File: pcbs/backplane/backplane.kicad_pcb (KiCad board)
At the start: 2 copper layers, 80 x 50 mm, 39 parts, among them P1 USB_B, P2 CONN_01X10, P3 CONN_02X03, P4 CONN_02X03, P5 CONN_02X07, P6 CONN_02X07, P7 CONN_01X03, P8 CONN_01X03, Q1 MMBT3904, Q2 MMBT3904, U1 LM358, U2 TC1262-33VDB, U3 LM358, U4 CH340G, Y1 Crystal

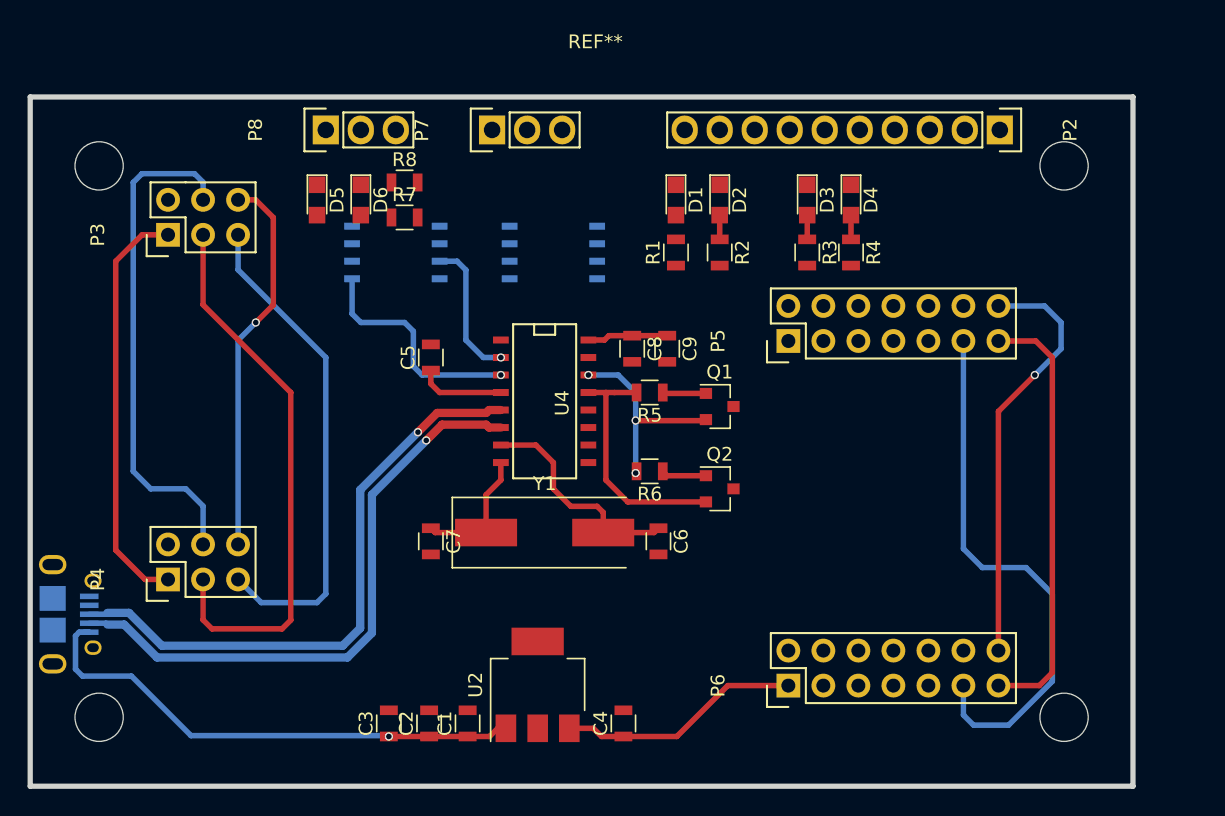
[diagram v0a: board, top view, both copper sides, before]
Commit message: Backplane version 1 ready.
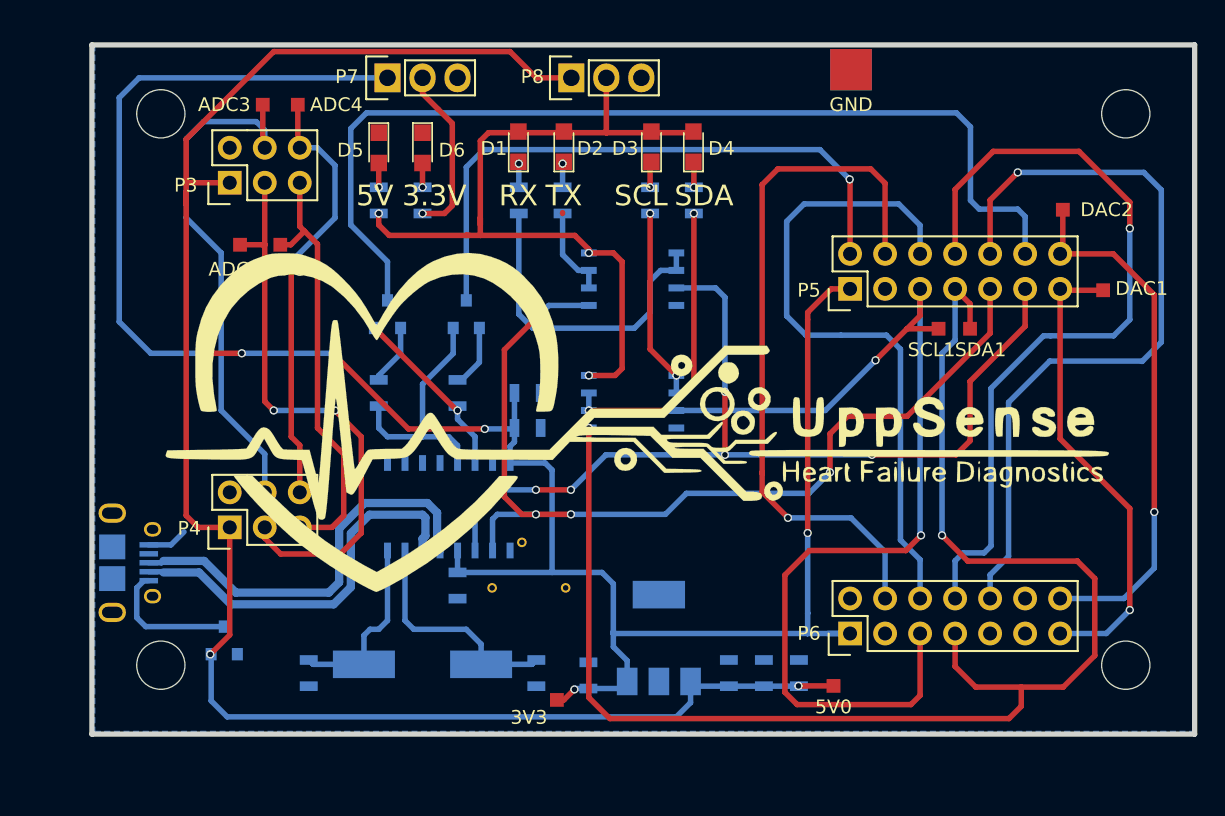
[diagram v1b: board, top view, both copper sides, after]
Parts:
- removed P2: CONN_01X10, mySamtec:Samtec-PHT-1-9-01-L-S
- added 3V3: TEST, myTestPoints:TP_SMD_quadr_1mm, F.Cu at (148.2, 113.7)
- added 5V0: TEST, myTestPoints:TP_SMD_quadr_1mm, F.Cu at (168.3, 112.7)
- added ADC1: TEST, myTestPoints:TP_SMD_quadr_1mm, F.Cu at (125.2, 80.7)
- added ADC2: TEST, myTestPoints:TP_SMD_quadr_1mm, F.Cu at (128.1, 80.7)
- added ADC3: TEST, myTestPoints:TP_SMD_quadr_1mm, F.Cu at (126.9, 70.6)
- added ADC4: TEST, myTestPoints:TP_SMD_quadr_1mm, F.Cu at (129.4, 70.6)
- added DAC1: TEST, myTestPoints:TP_SMD_quadr_1mm, F.Cu at (187.8, 84.0)
- added DAC2: TEST, myTestPoints:TP_SMD_quadr_1mm, F.Cu at (184.9, 78.2)
- added G***: LOGO, myPics:uppsense_logo, F.Cu at (153.8, 93.4)
- added G***: LOGO, myPics:uu_logo, B.Cu at (176.7, 92.8)
- added GND, GND1: TEST, myTestPoints:TP_SMD_quadr_3mm, F.Cu at (169.5, 68.0)
- added Q3: Si2323, TO_SOT_Packages_SMD:SOT-23, B.Cu at (124.1, 109.4)
- added REF**: Stitching-Via-0.5-0.7, myVias:Stitchging-Via-0.4-0.7, F.Cu at (148.8, 105.6)
- added REF**: Stitching-Via-0.5-0.7, myVias:Stitchging-Via-0.4-0.7, F.Cu at (143.5, 105.6)
- added REF**: Stitching-Via-0.5-0.7, myVias:Stitchging-Via-0.4-0.7, F.Cu at (145.7, 102.3)
- added SCL1: TEST, myTestPoints:TP_SMD_quadr_1mm, F.Cu at (175.9, 86.8)
- added SDA1: TEST, myTestPoints:TP_SMD_quadr_1mm, F.Cu at (178.2, 86.8)
- C1, C2, C3, C4, C5, C6, C7, C8, C9, Q1, Q2, R1, R2, R3, R4, R5, R6, R7, R8, U2, U4, Y1: moved to B.Cu
- moved Q1 25.0 mm to (135.9, 85.8), turned to 90 degrees
- moved C3 24.9 mm to (160.7, 111.8)
- moved C2 24.6 mm to (163.2, 111.8)
- moved C1 24.3 mm to (165.8, 111.8)
- moved Q2 22.3 mm to (141.6, 85.8), turned to 90 degrees
- moved R5 19.7 mm to (135.3, 91.5), turned to 270 degrees
- moved P8 18.2 mm to (149.3, 68.6)
- moved U1 17.3 mm to (153.7, 83.2)
- moved C5 16.7 mm to (141.0, 105.4), turned to 270 degrees
- moved R6 15.1 mm to (141.0, 91.5), turned to 270 degrees
- moved C7 13.0 mm to (130.2, 111.8)
- moved C6 13.0 mm to (146.7, 111.8)
- moved Y1 13.0 mm to (138.5, 111.2)
- moved U3 12.3 mm to (153.7, 92.1)
- moved D1 12.1 mm to (145.4, 73.6), turned to 90 degrees
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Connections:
- D1 pad 1: LED_5V -> Net-(D1-Pad1)
- D1 pad 2: Net-(D1-Pad2) -> LED_5V
- D2 pad 1: LED_5V -> Net-(D2-Pad1)
- D2 pad 2: Net-(D2-Pad2) -> LED_5V
- D3 pad 1: LED_5V -> Net-(D3-Pad1)
- D3 pad 2: Net-(D3-Pad2) -> LED_5V
- D4 pad 1: LED_5V -> Net-(D4-Pad1)
- D4 pad 2: Net-(D4-Pad2) -> LED_5V
- P1 pad 1: 5V -> Net-(P1-Pad1)
- P6 pad 11: UART_RX -> (no net)
- P6 pad 12: nRST -> (no net)
- P6 pad 2: GPIO0 -> (no net)
- P6 pad 9: UART_TX -> (no net)
- R1 pad 1: Net-(D1-Pad2) -> Net-(D1-Pad1)
- R2 pad 1: Net-(D2-Pad2) -> Net-(D2-Pad1)
- R3 pad 1: Net-(D3-Pad2) -> Net-(D3-Pad1)
- R4 pad 1: Net-(D4-Pad2) -> Net-(D4-Pad1)
- U4 pad 2: UART_RX -> UART_TX
- U4 pad 3: UART_TX -> UART_RX
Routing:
- net 3.3V: track 29.8 -> 157.5 mm, vias 0 -> 6
- net I2C_SDA: track 0.00 -> 107.0 mm, vias 0 -> 2
- net I2C_SCL: track 0.00 -> 77.2 mm, vias 0 -> 2
- net nRST: track 0.00 -> 71.9 mm
- net 5V: track 67.7 -> 127.3 mm, vias 1 -> 2
- net GPIO3: track 0.00 -> 58.6 mm, vias 0 -> 1
- net LED_5V: track 0.00 -> 57.8 mm, vias 0 -> 3
- net GPIO4: track 0.00 -> 56.4 mm, vias 0 -> 1
- net UART_TX: track 16.7 -> 69.8 mm, vias 1 -> 4
- net GPIO1: track 0.00 -> 51.3 mm, vias 0 -> 1
- net GPIO2: track 0.00 -> 47.7 mm
- net GPIO0: track 0.00 -> 44.3 mm, vias 0 -> 1
- net Net-(R1-Pad2): track 0.00 -> 23.5 mm
- net Net-(R4-Pad2): track 0.00 -> 22.0 mm, vias 0 -> 2
- net UART_RX: track 49.7 -> 68.9 mm, vias 1 -> 5
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- added copper zone on B.Cu, net GND
- added copper zone on F.Cu, net GND
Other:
- board text added: "3.3V"
- board text added: "5V"
- board text added: "RX"
- board text added: "SCL"
- board text added: "SDA"
- board text added: "TX"

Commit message: Simulated a lot today. Ideas for the new transimpedance amp. are there.
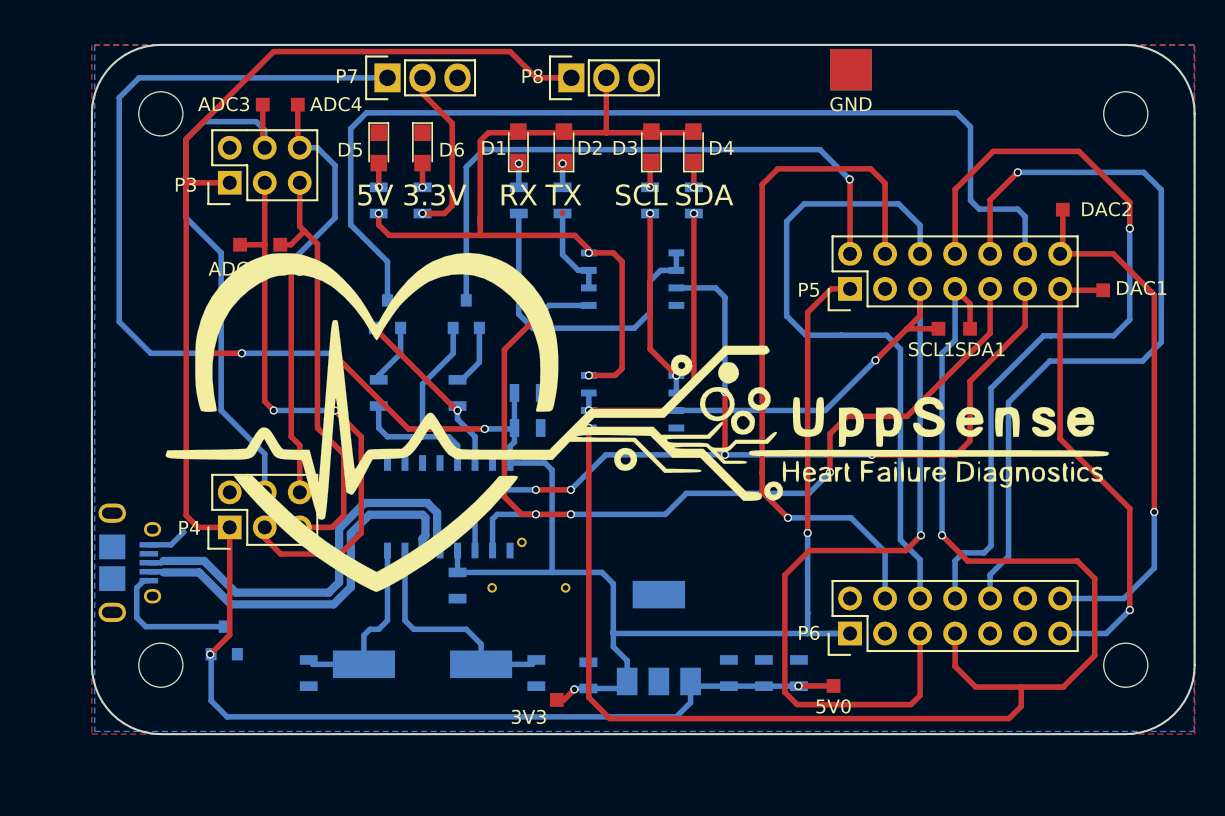
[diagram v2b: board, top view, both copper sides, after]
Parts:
- removed the REF** at (114.5, 116.2)
- added REF**: MountingHole_3.2mm_M3_DIN965, Mounting_Holes:MountingHole_3.2mm_M3_DIN965, F.Cu at (189.5, 111.2)
- added REF**: MountingHole_3.2mm_M3_DIN965, Mounting_Holes:MountingHole_3.2mm_M3_DIN965, F.Cu at (189.5, 71.2)
- added REF**: MountingHole_3.2mm_M3_DIN965, Mounting_Holes:MountingHole_3.2mm_M3_DIN965, F.Cu at (119.5, 71.2)
- added REF**: MountingHole_3.2mm_M3_DIN965, Mounting_Holes:MountingHole_3.2mm_M3_DIN965, F.Cu at (119.5, 111.2)
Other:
- outline, holes or cut-outs redrawn
